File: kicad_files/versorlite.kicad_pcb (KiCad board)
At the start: 4 copper layers, 33 x 81.3 mm, 136 parts, among them J1 Conn_01x01_Socket, J10 IGN_2, J3 RFD900ux 10 Pin Header, J4 Conn_ARM_JTAG_SWD_10, J5 RFD900ux 3 Pin Power Select, J6 USB_C_Receptacle_USB2.0_16P, J7 Micro_SD_Card_Det2, J8 Conn_01x02_Socket, J9 IGN_1, Q1 FDMC510P-MS, Q2 AO3400A, Q3 AO3400A, SW1 SW_Push, SW2 SW_Push, U1 STM32F407VGTx, U10 W25Q128JVS, U11 LT1963AxST-3.3, U12 AP63205WU, U13 74LVC1G125, U2 MS5611-01BA, U3 BMI088, U4 MMC5983MA, U5 MAX-M10S, U6 BMP388, U7 LSM6DSM, U9 WE-TVS-82400102, Y1 LFXTAL036869Reel 8MHz Crystal

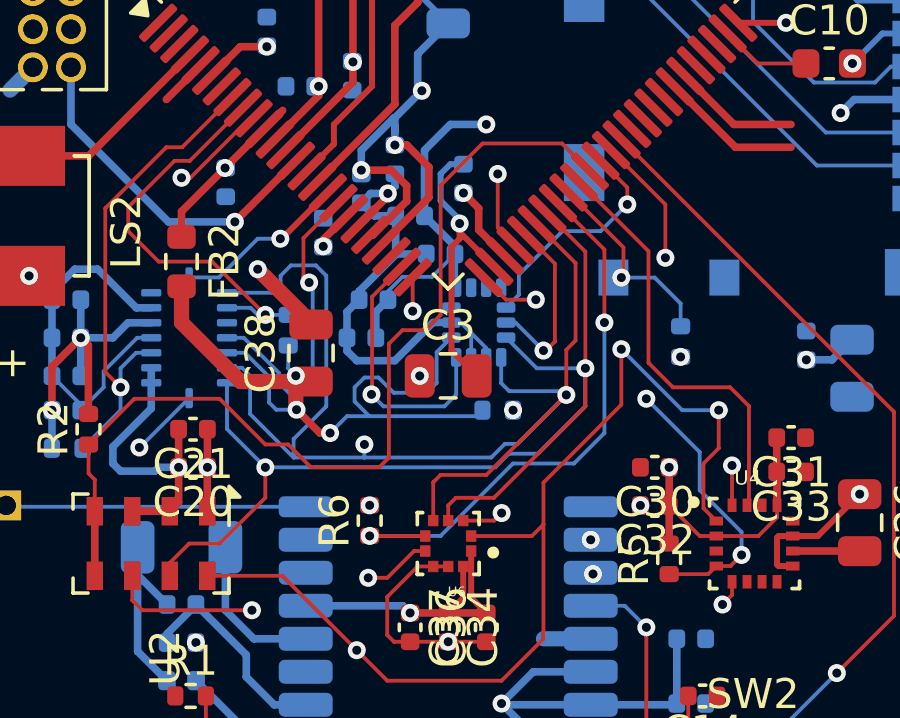
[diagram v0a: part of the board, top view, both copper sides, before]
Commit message: Rearrange
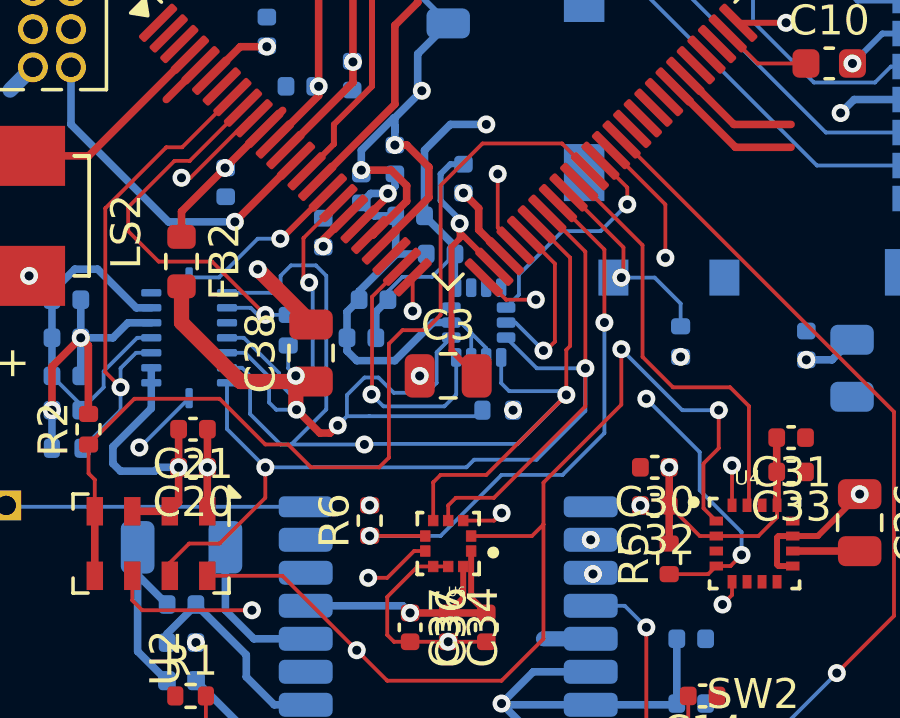
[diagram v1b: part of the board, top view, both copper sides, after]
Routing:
- net /MCU/SPI1_MISO: track 63.6 -> 62.3 mm
